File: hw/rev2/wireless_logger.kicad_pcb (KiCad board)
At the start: 4 copper layers, 137 parts, among them J1 FCI 10118194, J2 CONN_2, J3 SSD1306_SER, J4 SWD_10PIN, J5 CONN_5, P1 CONN_6X2, Q1 2N7002P, Q2 2N7002P, U1 MT29FXX01A, U10 CC2541, U11 STM32F40X_BGA176, U2 MAG3110, U3 MMA8452Q, U4 LPS331AP, U5 L3GD20, U6 MCP111T-315, U7 BQ24095, U8 TPS62698, U9 CC1101, X1 FA-128 26.0000MF10Z-W3, X2 9HT10-32.768KBZF-T, X3 FA-128 32.0000MF20X-K3, X4 XRCGB25M000F0L00R0, X5 9HT10-32.768KBZF-T

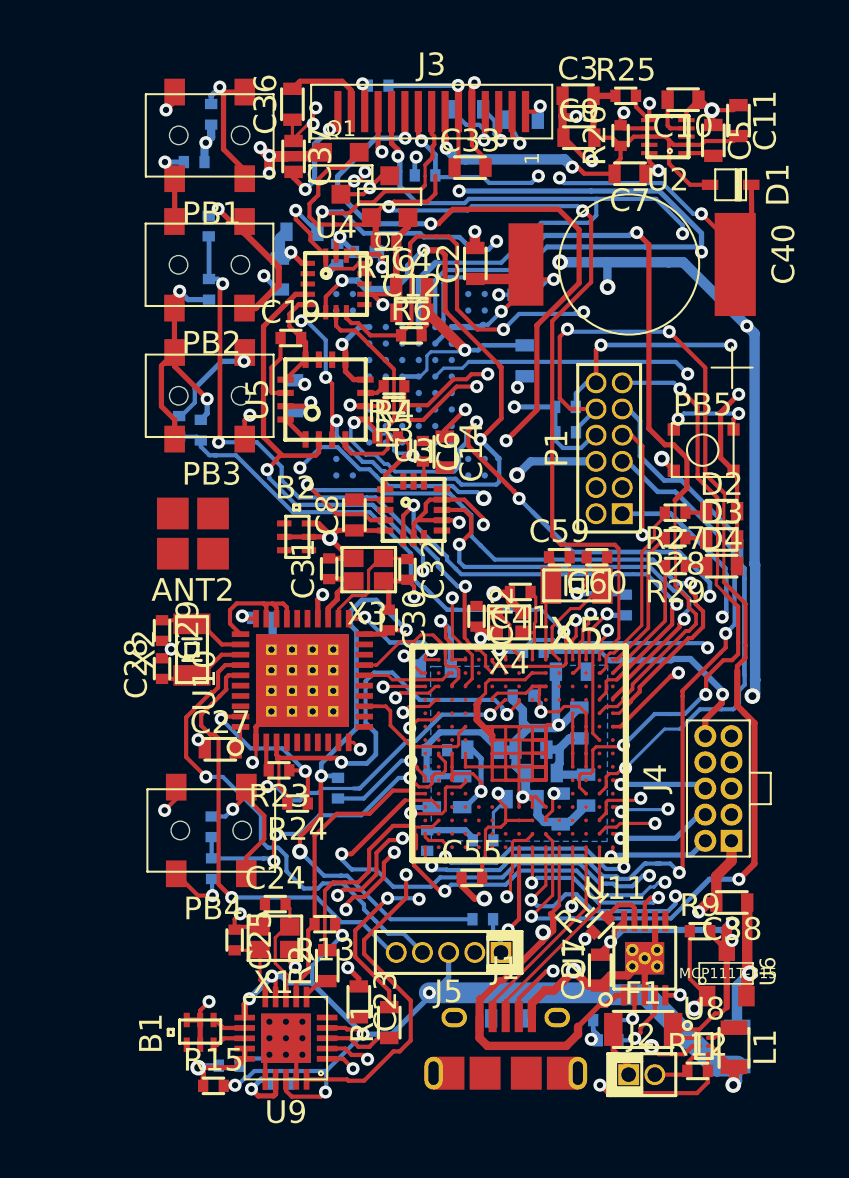
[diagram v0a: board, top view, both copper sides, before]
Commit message: Ready for first schematic review
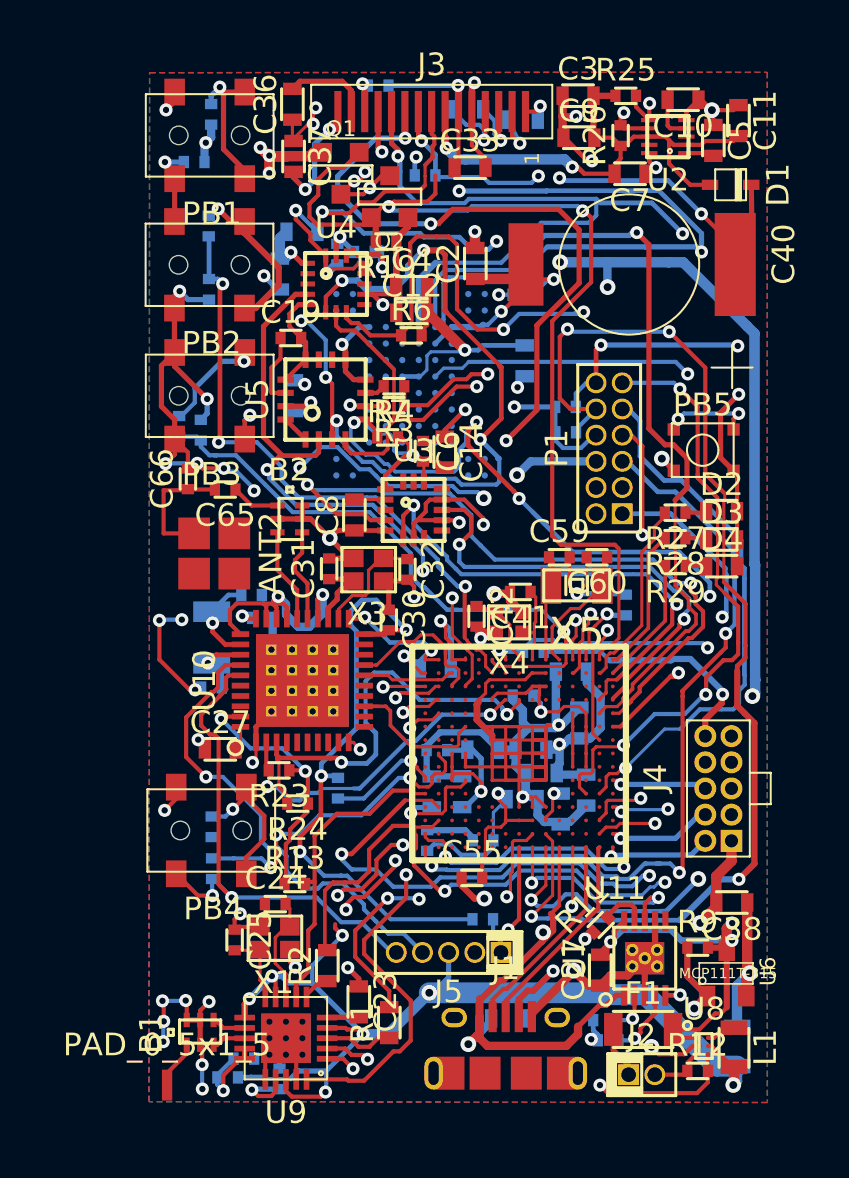
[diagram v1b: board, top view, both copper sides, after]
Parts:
- added C65: CAP, SMD0402, F.Cu at (173.7, 130.3)
- added C66: CAP, SMD0402, F.Cu at (171.9, 129.8)
- added PAD_0_5x1_5: VAL**, PAD_0_5x1_5, F.Cu at (170.9, 159.2)
- C28, C29, R15, X2: moved to B.Cu
- C61, C62, C63, C64: value 10n -> 100n
- R30, R31, R32, R33: value 470k -> 3.3k
- moved C29 4.67 mm to (175.0, 135.4), turned to 0 degrees
- moved C28 2.57 mm to (173.0, 139.9), turned to 180 degrees
- moved R13 2.44 mm to (177.1, 149.4), turned to 0 degrees
- moved ANT2 1.41 mm to (173.2, 133.4), turned to 270 degrees
- moved X2 1.12 mm to (173.0, 137.4)
- moved B2 0.93 mm to (176.8, 131.7)
- moved R9 0.81 mm to (196.6, 152.5)
- moved R15 0.80 mm to (173.8, 158.8)
- moved C26 0.79 mm to (174.6, 157.9)
- moved R14 0.23 mm to (176.3, 158.9), turned to 270 degrees
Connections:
- B2 pad 1: /Bluetooth/BT_ANT_SE -> N-00000226
- R33 pad 2: /STM32F4/EXTI8 -> (no net)
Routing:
- net V3: track 277.3 -> 306.4 mm, vias 28 -> 29
- net GND: track 266.7 -> 284.0 mm, vias 47 -> 59
- net /Bluetooth/BT_ANT_SE: track 0.00 -> 6.09 mm
- net /Bluetooth/BT_ANT_DP: track 0.00 -> 4.59 mm
- net /Bluetooth/BT_ANT_DN: track 0.00 -> 4.59 mm
- net /STM32F4/I2C3_SCL: track 55.9 -> 51.9 mm
- net Vbus: track 50.8 -> 54.1 mm, vias 2 -> 3
- net /STM32F4/REG_nUSB_CONN: track 19.6 -> 16.5 mm
- net N-00000194: track 0.00 -> 2.44 mm
- net N-00000226: track 0.00 -> 2.36 mm
- net N-00000199: track 0.00 -> 1.54 mm
- net Vbat: track 92.3 -> 90.8 mm, vias 8 -> 7
- net N-00000216: track 4.29 -> 3.32 mm, vias 0 -> 1
- net N-00000189: track 9.87 -> 9.13 mm
- net /STM32F4/EXTI8: track 16.5 -> 15.8 mm
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- added copper zone on F.Cu, net GND
